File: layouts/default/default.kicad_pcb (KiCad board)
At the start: 2 copper layers, 10 parts

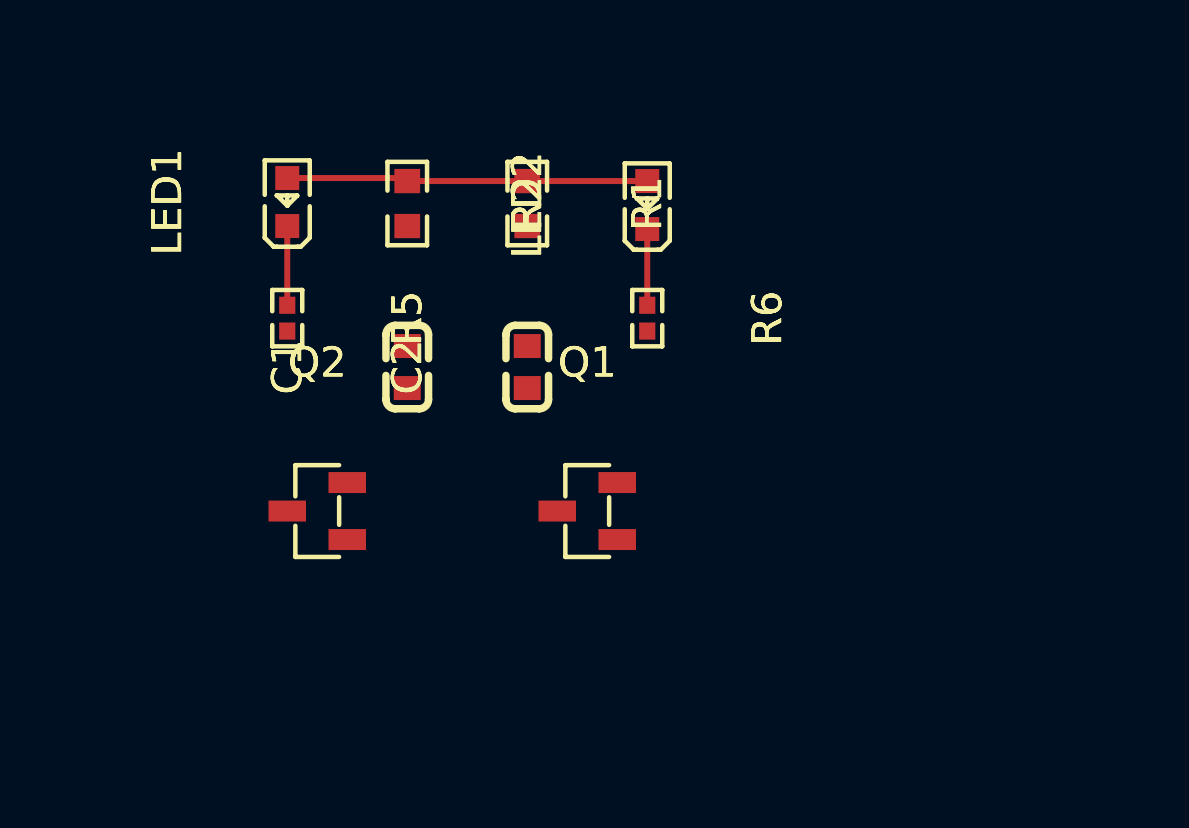
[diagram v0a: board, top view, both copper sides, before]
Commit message: Wild stuff
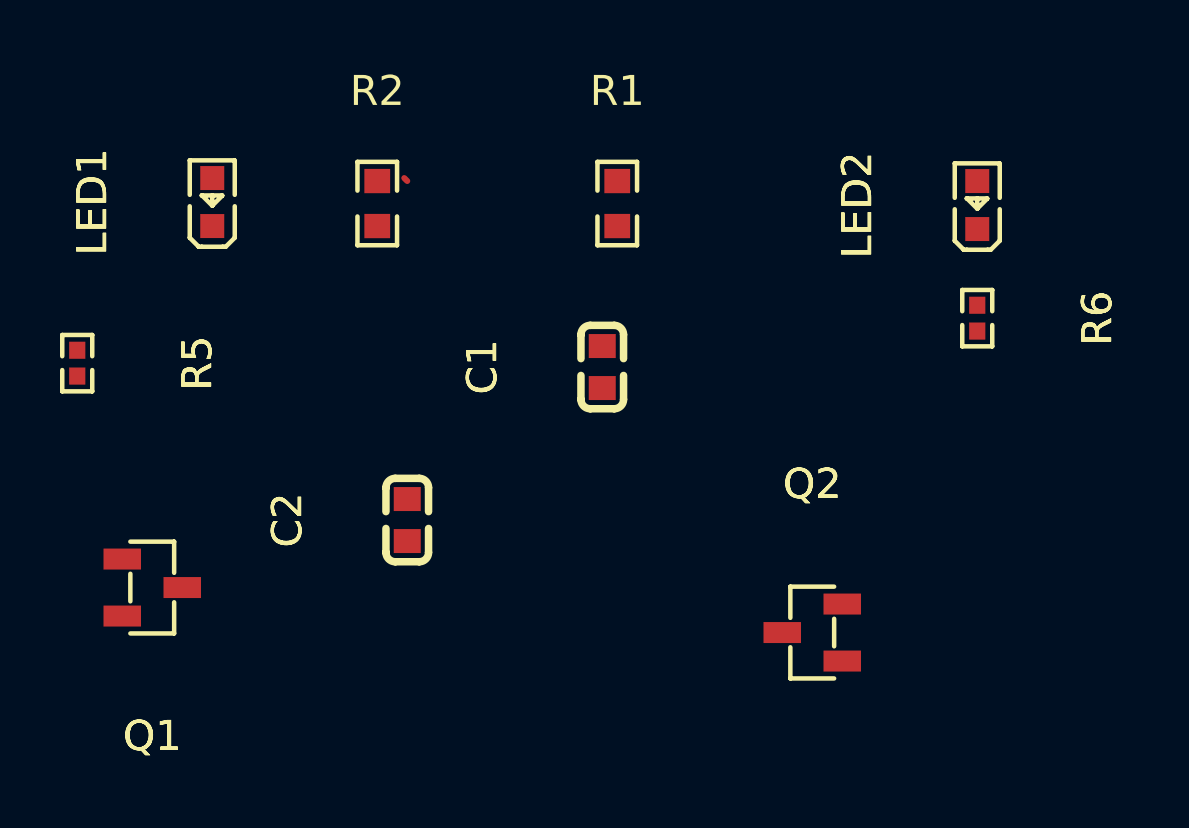
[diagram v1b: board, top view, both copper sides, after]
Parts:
- moved Q2 17.0 mm to (-16.0, -26.4)
- moved Q1 14.7 mm to (-38.0, -27.9), turned to 180 degrees
- moved LED2 11.0 mm to (-10.5, -40.7)
- moved R6 11.0 mm to (-10.5, -36.9)
- moved R5 7.16 mm to (-40.5, -35.4)
- moved C1 6.50 mm to (-23.0, -35.3)
- moved C2 6.48 mm to (-29.5, -30.2)
- moved R1 3.00 mm to (-22.5, -40.8)
- moved LED1 2.50 mm to (-36.0, -40.8)
- moved R2 1.00 mm to (-30.5, -40.8)
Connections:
- C1 pad 1: c1-C -> GND
- C2 pad 1: c2-C -> GND
- Q1 pad 3: c2-C -> GND
- Q2 pad 3: c1-C -> GND
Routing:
- net VIN_PAD: track 12.0 -> 0.14 mm
- net footprint-cathode-0: track 2.64 -> 0.00 mm
- net footprint-cathode-1: track 2.54 -> 0.00 mm
